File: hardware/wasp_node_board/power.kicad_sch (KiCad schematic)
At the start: 29 parts, among them J1 Conn_01x02, J7 USB_C_Receptacle_USB2.0_16P, SW1 C&K JS202011, U2 USBLC6-2SC6, U4 TPSM863253, U6 LP5907MFX-1.2

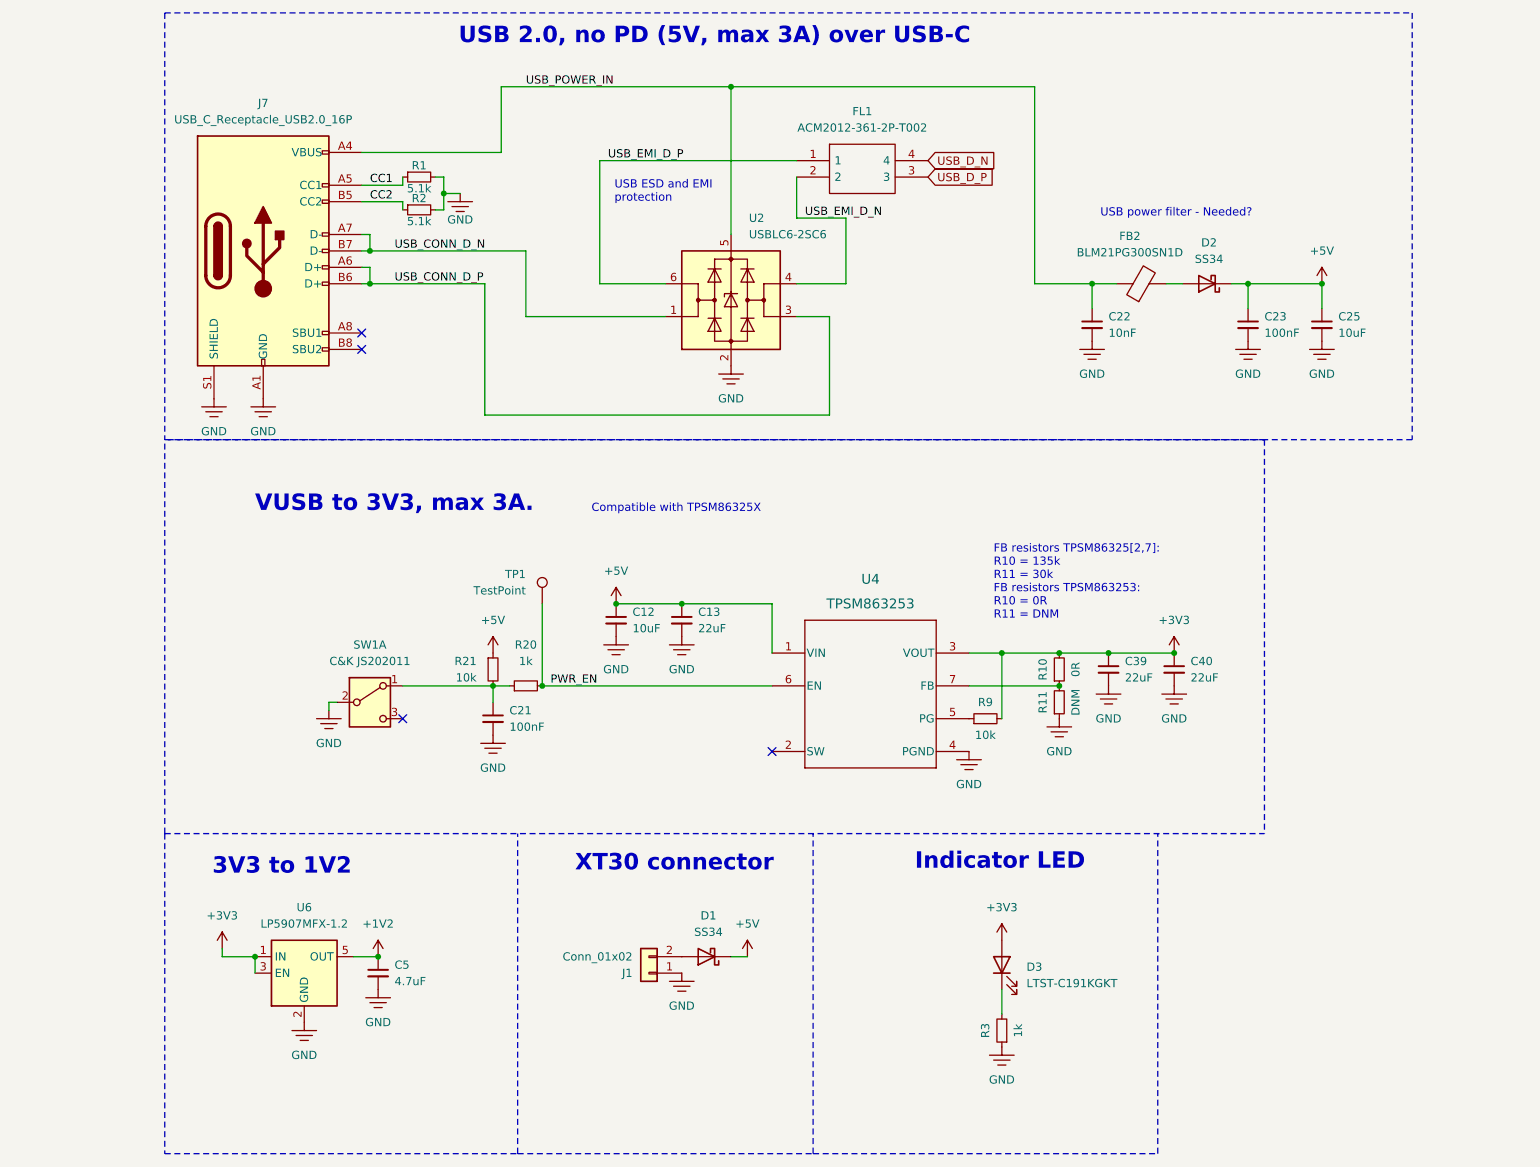
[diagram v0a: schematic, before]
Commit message: Schematic verified clean and layout started
Co-Authored-By: Claude Opus 5 <noreply@anthropic.com>
Claude-Session: https://claude.ai/code/session_01R5uaLk4w44r9dBy8LCo6if
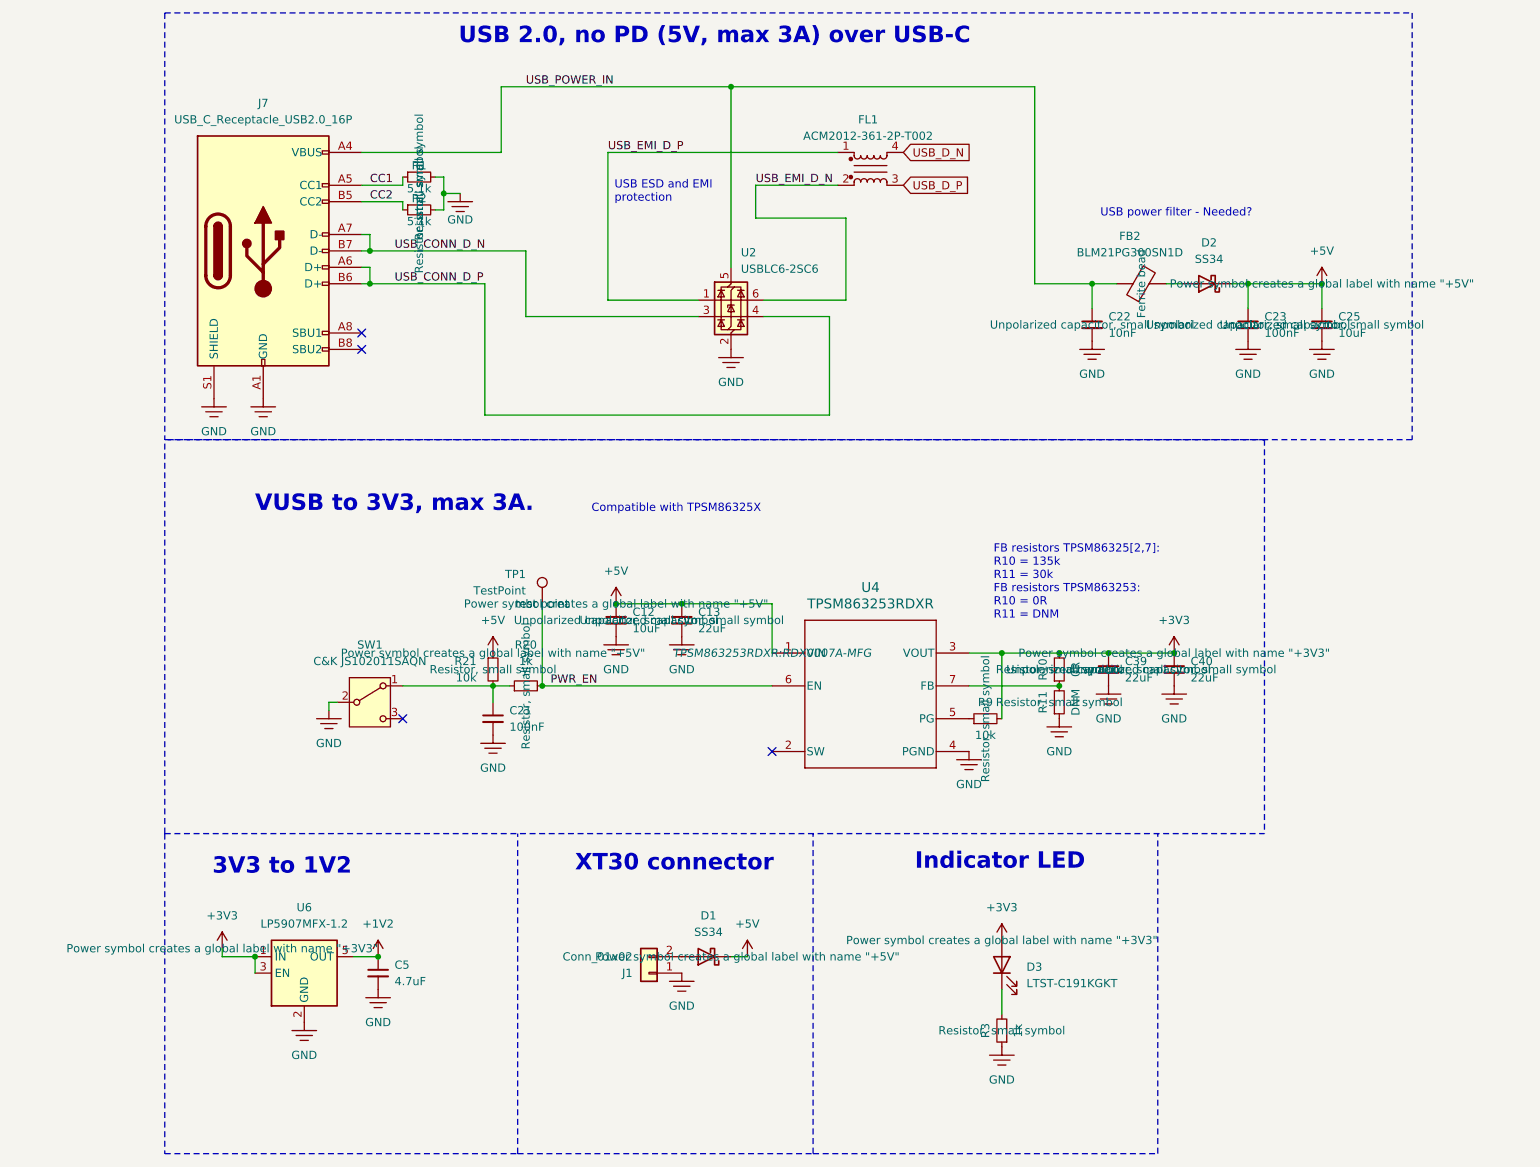
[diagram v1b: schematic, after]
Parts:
- removed FL1: ACM2012-361-2P-T002, ACM2012-361-2P-T002:ACM2012_TDK, symbol SamacSys_Parts:ACM2012-201-2P-T001
- removed SW1: C&K JS202011, Button_Switch_THT:SW_CK_JS202011CQN_DPDT_Straight, symbol Switch:SW_DPDT_x2
- removed U4: TPSM863253, TPSM863253RDXR:RDX0007A-MFG, symbol ul_PTPSM863252RDXR:PTPSM863252RDXR
- added FL1: ACM2012-361-2P-T002, ACM2012-361-2P-T002:ACM2012_TDK, symbol Filter:Choke_CommonMode_PulseElectronics_PH9455x105NL
- added SW1: C&K JS102011SAQN, Button_Switch_SMD:SW_SPDT_CK_JS102011SAQN, symbol Switch:SW_SPDT
- added U4: TPSM863253RDXR, TPSM863253RDXR:RDX0007A-MFG, symbol TPSM863253RDXR:TPSM863253RDXR
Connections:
- net +3V3: now also U4.3 (VOUT)
- net +5V: now also U4.1 (VIN)
- net GND: now also SW1.2 (B), U4.4 (PGND)
- net PWR_EN: now also U4.6 (EN)
- net USB_CONN_D_N: now also U2.3 (I/O2); no longer U2.1 (I/O1)
- net USB_CONN_D_P: now also U2.4 (I/O2); no longer U2.3 (I/O2)
- net USB_D_N: now also FL1.4
- net USB_D_P: now also FL1.3
- net USB_EMI_D_N: now also U2.6 (I/O1), FL1.2; no longer U2.4 (I/O2)
- net USB_EMI_D_P: now also U2.1 (I/O1), FL1.1; no longer U2.6 (I/O1)
- net at R10.1, R11.2: now also U4.7 (FB)
- net at C21.1, R20.1, R21.2: now also SW1.1 (A)
- net at R9.1: now also U4.5 (PG)
